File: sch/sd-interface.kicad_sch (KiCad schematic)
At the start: 33 parts, among them J15 F32Q-1A7H1-11022, J16 MEM2075-00-140-01-A, J17 5V_out, J19 3V3_in, Q1 Q_PMOS_GSD, U10 CD4043BDR, U11 TPS22919DCKR, U8 MAX4996LETG_

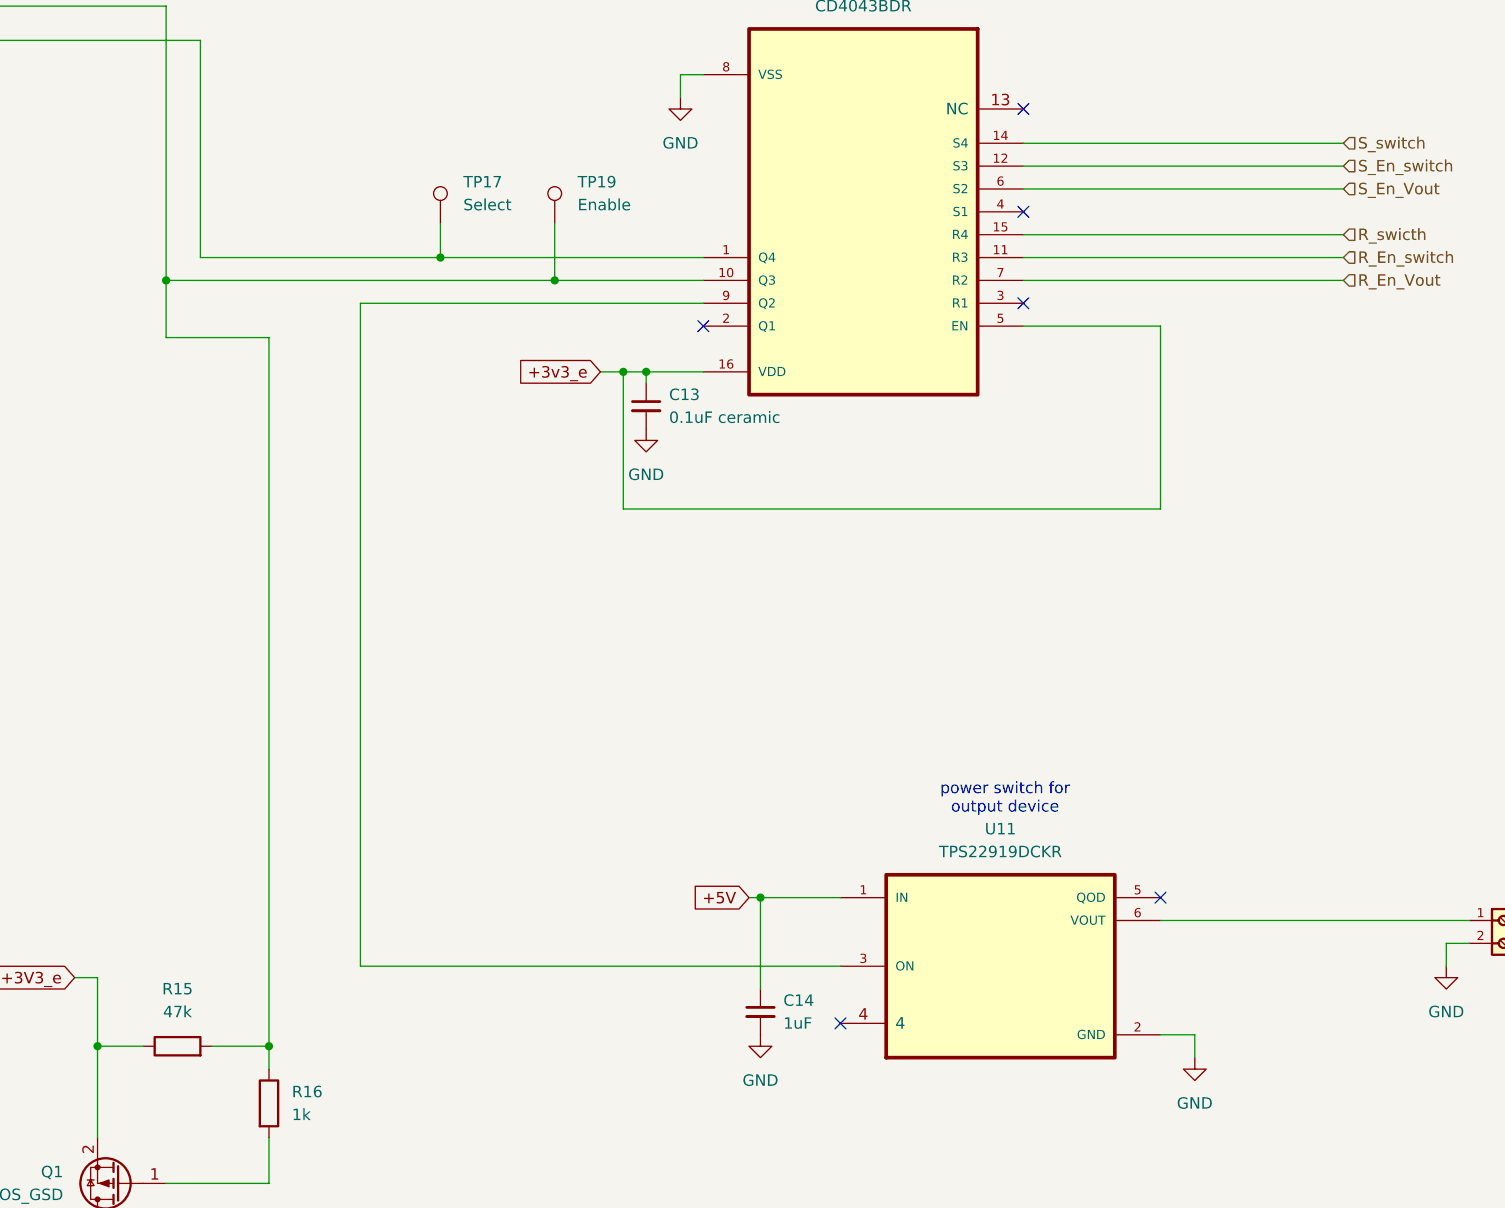
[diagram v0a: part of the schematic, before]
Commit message: started pcb design
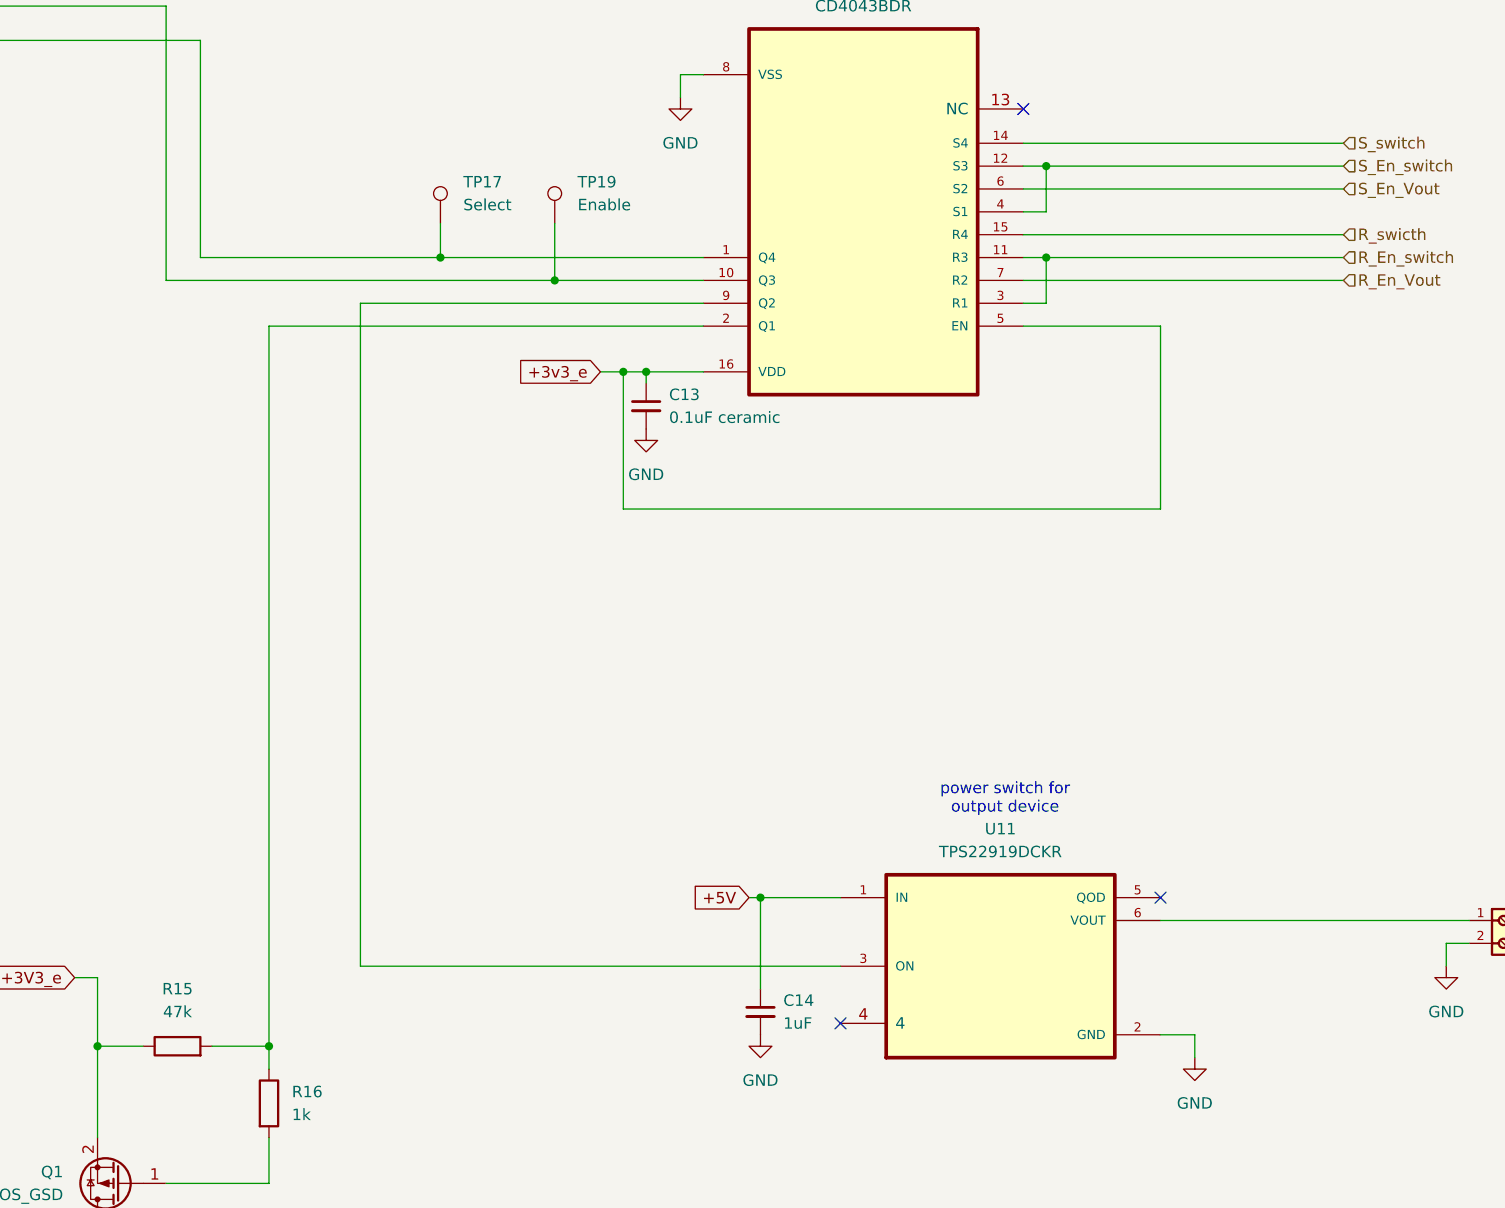
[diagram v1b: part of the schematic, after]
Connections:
- net R_En_switch: now also U10.3 (R1)
- net S_En_switch: now also U10.4 (S1)
- net at TP19.1, U10.10 (Q3), U8.15 (EN): no longer R15.2, R16.1
- net at U10.2 (Q1): now also R15.2, R16.1
- no-connect marks 7 -> 4
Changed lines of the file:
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@@
+	)
+	(junction
+		(at 302.26 132.08)
+		(diameter 0)
+		(color 0 0 0 0)
 	)
 	(junction
@@
 	)
 	(junction
-		(at 204.47 144.78)
+		(at 302.26 142.24)
 		(diameter 0)
 		(color 0 0 0 0)
@@
 	)
 	(no_connect
-		(at 299.72 147.32)
-	)
-	(no_connect
 		(at 299.72 125.73)
 	)
@@
 	)
 	(no_connect
-		(at 299.72 137.16)
-	)
-	(no_connect
 		(at 279.4 227.33)
 	)
@@
 		(at 175.26 266.7)
 	)
-	(no_connect
-		(at 264.16 149.86)
-	)
 	(wire
 		(pts
@@
 	(wire
 		(pts
+			(xy 299.72 137.16) (xy 302.26 137.16)
+		)
+		(stroke
+			(width 0)
+			(type default)
+		)
+	)
+	(wire
+		(pts
 			(xy 152.4 66.04) (xy 152.4 69.85)
 		)
@@
 	(wire
 		(pts
-			(xy 204.47 151.13) (xy 204.47 144.78)
-		)
-		(stroke
-			(width 0)
-			(type default)
-		)
-	)
-	(wire
-		(pts
 			(xy 234.95 73.66) (xy 234.95 62.23)
 		)
@@
 	(wire
 		(pts
+			(xy 302.26 132.08) (xy 335.28 132.08)
+		)
+		(stroke
+			(width 0)
+			(type default)
+		)
+	)
+	(wire
+		(pts
 			(xy 99.06 163.83) (xy 99.06 190.5)
 		)
@@
 	(wire
 		(pts
-			(xy 299.72 142.24) (xy 335.28 142.24)
+			(xy 299.72 142.24) (xy 302.26 142.24)
 		)
 		(stroke
@@
 	(wire
 		(pts
+			(xy 215.9 149.86) (xy 215.9 229.87)
+		)
+		(stroke
+			(width 0)
+			(type default)
+		)
+	)
+	(wire
+		(pts
 			(xy 71.12 87.63) (xy 71.12 123.19)
 		)
@@
 	(wire
 		(pts
-			(xy 215.9 151.13) (xy 204.47 151.13)
-		)
-		(stroke
-			(width 0)
-			(type default)
-		)
-	)
-	(wire
-		(pts
 			(xy 346.71 218.44) (xy 346.71 220.98)
 		)
@@
 	(wire
 		(pts
-			(xy 215.9 229.87) (xy 215.9 151.13)
-		)
-		(stroke
-			(width 0)
-			(type default)
-		)
-	)
-	(wire
-		(pts
 			(xy 111.76 36.83) (xy 111.76 50.8)
 		)
@@
 	(wire
 		(pts
+			(xy 302.26 142.24) (xy 335.28 142.24)
+		)
+		(stroke
+			(width 0)
+			(type default)
+		)
+	)
+	(wire
+		(pts
+			(xy 264.16 149.86) (xy 215.9 149.86)
+		)
+		(stroke
+			(width 0)
+			(type default)
+		)
+	)
+	(wire
+		(pts
 			(xy 207.01 62.23) (xy 234.95 62.23)
 		)
@@
 	(wire
 		(pts
+			(xy 302.26 142.24) (xy 302.26 147.32)
+		)
+		(stroke
+			(width 0)
+			(type default)
+		)
+	)
+	(wire
+		(pts
 			(xy 96.52 36.83) (xy 99.06 36.83)
 		)
@@
 	(wire
 		(pts
-			(xy 299.72 132.08) (xy 335.28 132.08)
+			(xy 299.72 132.08) (xy 302.26 132.08)
 		)
 		(stroke
@@
 	(wire
 		(pts
+			(xy 302.26 137.16) (xy 302.26 132.08)
+		)
+		(stroke
+			(width 0)
+			(type default)
+		)
+	)
+	(wire
+		(pts
 			(xy 130.81 203.2) (xy 173.99 203.2)
 		)
@@
 		)
 		(stroke
+			(width 0)
+			(type default)
+		)
+	)
+	(wire
+		(pts
+			(xy 302.26 147.32) (xy 299.72 147.32)
+		)
+		(stroke

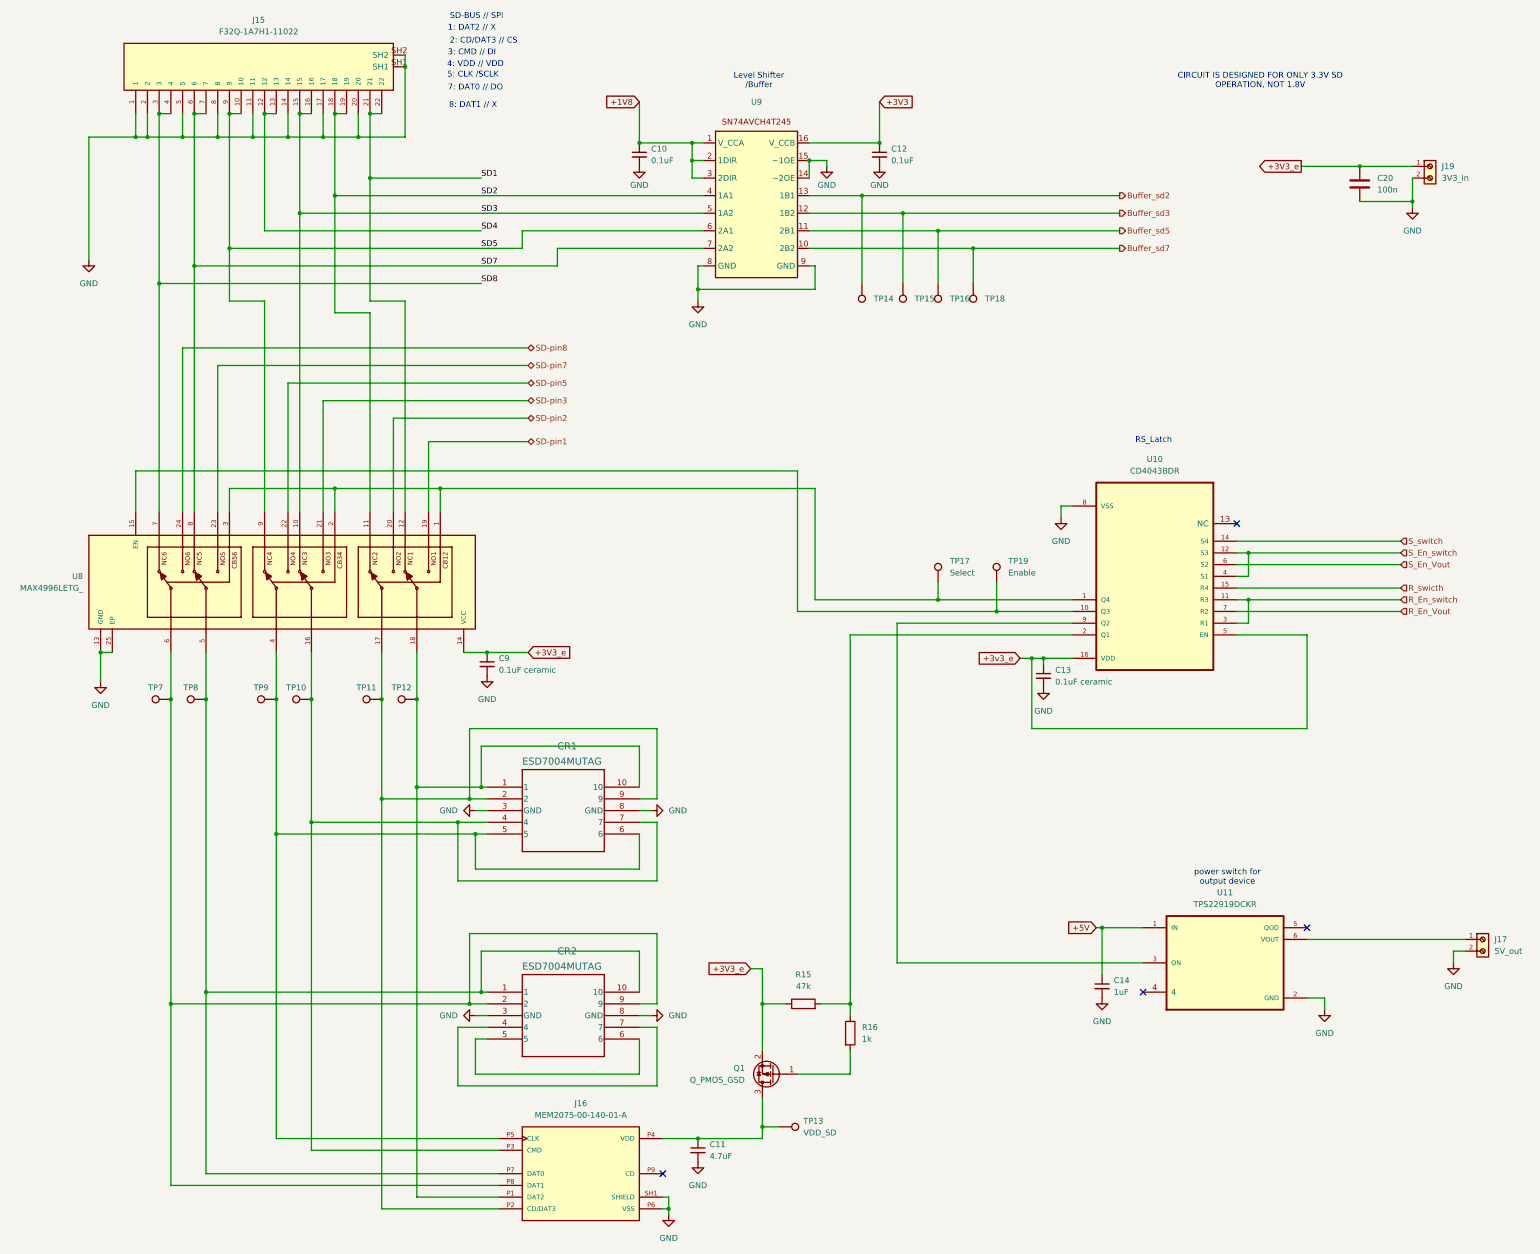
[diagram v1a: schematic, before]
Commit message: work pcb about 70 percent
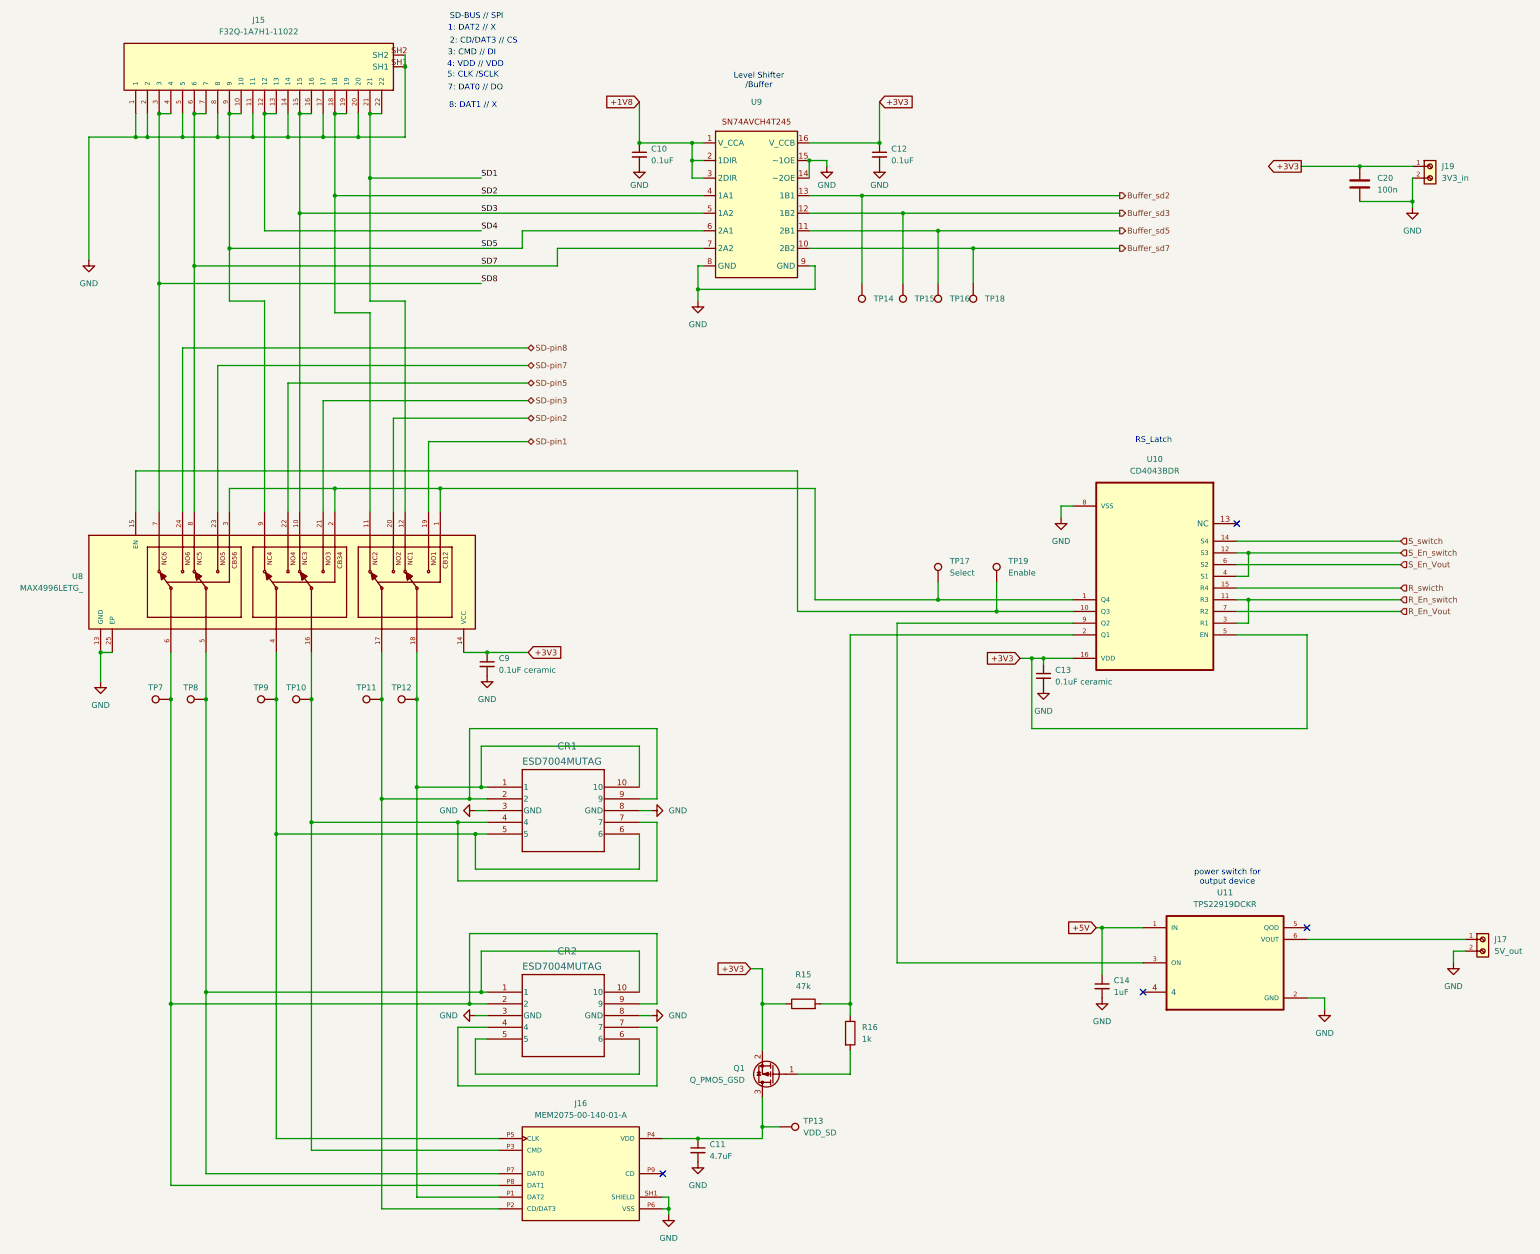
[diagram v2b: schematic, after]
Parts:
- TP10, TP11, TP12, TP7, TP8, TP9: footprint TestPoint:TestPoint_Loop_D2.50mm_Drill1.85mm -> TestPoint:TestPoint_Pad_D1.0mm
- TP13, TP14, TP15, TP16, TP17, TP18, TP19: footprint TestPoint:TestPoint_Loop_D2.50mm_Drill1.85mm -> TestPoint:TestPoint_Loop_D2.60mm_Drill1.6mm_Beaded
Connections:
- net +3V3_e is gone; now on net +3V3: C20.1, C9.1, J19.1, Q1.2 (S), R15.1, U8.14 (VCC)
- net +3v3_e is gone; now on net +3V3: C13.1, U10.16 (VDD), U10.5 (EN)
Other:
- note removed: "CIRCUIT IS DESIGNED FOR ONLY 3.3V SD OPERATION, NOT 1.8V"
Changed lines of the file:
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@@
 		)
 	)
-	(text "CIRCUIT IS DESIGNED FOR ONLY 3.3V SD \nOPERATION, NOT 1.8V"
-		(exclude_from_sim no)
-		(at 304.8 29.718 0)
-		(effects
-			(font
-				(size 1.27 1.27)
-			)
-		)
-	)
 	(text "8: DAT1 // X"
 		(exclude_from_sim no)
@@
 		)
 	)
-	(global_label "+3V3_e"
+	(global_label "+3V3"
 		(shape input)
 		(at 146.05 153.67 0)
@@
 		)
 		(property "Intersheetrefs" "${INTERSHEET_REFS}"
-			(at 156.1714 153.67 0)
+			(at 154.1152 153.67 0)
 			(effects
 				(font
@@
 		)
 	)
-	(global_label "+3V3_e"
+	(global_label "+3V3"
 		(shape input)
 		(at 194.31 222.25 180)
@@
 		)
 	)
-	(global_label "+3v3_e"
+	(global_label "+3V3"
 		(shape input)
 		(at 252.73 154.94 180)
@@
 		)
 		(property "Intersheetrefs" "${INTERSHEET_REFS}"
-			(at 246.3582 154.94 0)
+			(at 244.6648 154.94 0)
 			(effects
 				(font
@@
 		)
 	)
-	(global_label "+3V3_e"
+	(global_label "+3V3"
 		(shape output)
 		(at 313.69 48.26 180)
@@
 		)
 		(property "Intersheetrefs" "${INTERSHEET_REFS}"
-			(at 303.5686 48.26 0)
+			(at 305.6248 48.26 0)
 			(effects
 				(font
@@
 			)
 		)
-		(property "Footprint" "TestPoint:TestPoint_Loop_D2.50mm_Drill1.85mm"
+		(property "Footprint" "TestPoint:TestPoint_Loop_D2.60mm_Drill1.6mm_Beaded"
 			(at 213.36 73.66 0)
 			(effects
@@
 			)
 		)
-		(property "Footprint" "TestPoint:TestPoint_Loop_D2.50mm_Drill1.85mm"
+		(property "Footprint" "TestPoint:TestPoint_Loop_D2.60mm_Drill1.6mm_Beaded"
 			(at 200.66 261.62 0)
 			(effects
@@
 			)
 		)
-		(property "Footprint" "TestPoint:TestPoint_Loop_D2.50mm_Drill1.85mm"
+		(property "Footprint" "TestPoint:TestPoint_Pad_D1.0mm"
 			(at 76.2 158.75 0)
 			(effects
@@
 			)
 		)
-		(property "Footprint" "TestPoint:TestPoint_Loop_D2.50mm_Drill1.85mm"
+		(property "Footprint" "TestPoint:TestPoint_Loop_D2.60mm_Drill1.6mm_Beaded"
 			(at 222.25 73.66 0)
 			(effects
@@
 			)
 		)
-		(property "Footprint" "TestPoint:TestPoint_Loop_D2.50mm_Drill1.85mm"
+		(property "Footprint" "TestPoint:TestPoint_Loop_D2.60mm_Drill1.6mm_Beaded"
 			(at 252.73 138.43 0)
 			(effects
@@
 			)
 		)
-		(property "Footprint" "TestPoint:TestPoint_Loop_D2.50mm_Drill1.85mm"
+		(property "Footprint" "TestPoint:TestPoint_Pad_D1.0mm"
 			(at 91.44 158.75 0)
 			(effects
@@
 			)
 		)
-		(property "Footprint" "TestPoint:TestPoint_Loop_D2.50mm_Drill1.85mm"
+		(property "Footprint" "TestPoint:TestPoint_Loop_D2.60mm_Drill1.6mm_Beaded"
 			(at 229.87 73.66 0)
 			(effects
@@
 			)
 		)
-		(property "Footprint" "TestPoint:TestPoint_Loop_D2.50mm_Drill1.85mm"
+		(property "Footprint" "TestPoint:TestPoint_Loop_D2.60mm_Drill1.6mm_Beaded"
 			(at 240.03 138.43 0)
 			(effects
@@
 			)
 		)
-		(property "Footprint" "TestPoint:TestPoint_Loop_D2.50mm_Drill1.85mm"
+		(property "Footprint" "TestPoint:TestPoint_Pad_D1.0mm"
 			(at 114.3 158.75 0)
 			(effects
@@
 			)
 		)
-		(property "Footprint" "TestPoint:TestPoint_Loop_D2.50mm_Drill1.85mm"
+		(property "Footprint" "TestPoint:TestPoint_Loop_D2.60mm_Drill1.6mm_Beaded"
 			(at 237.49 73.66 0)
 			(effects
@@
 			)
 		)
-		(property "Footprint" "TestPoint:TestPoint_Loop_D2.50mm_Drill1.85mm"
+		(property "Footprint" "TestPoint:TestPoint_Pad_D1.0mm"
 			(at 121.92 158.75 0)
 			(effects
@@
 			)
 		)
-		(property "Footprint" "TestPoint:TestPoint_Loop_D2.50mm_Drill1.85mm"
+		(property "Footprint" "TestPoint:TestPoint_Pad_D1.0mm"
 			(at 68.58 158.75 0)
 			(effects
@@
 			)
 		)
-		(property "Footprint" "TestPoint:TestPoint_Loop_D2.50mm_Drill1.85mm"
+		(property "Footprint" "TestPoint:TestPoint_Pad_D1.0mm"
 			(at 99.06 158.75 0)
 			(effects
